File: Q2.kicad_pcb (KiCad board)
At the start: 2 copper layers, 86 x 55 mm, 167 parts, among them U1 LM317, U10 SP-2U1+, U11 SMA, U12 LT1009, U13 TL974, U14 PMA4-33GLN+, U2 Teensy3.2, U3 SMA, U4 ROS-2536C-119+, U5 PMA4-33GLN+, U6 PGA-103+, U7 TCBT-14+, U8 SIM-43LH+, U9 GAT-7+

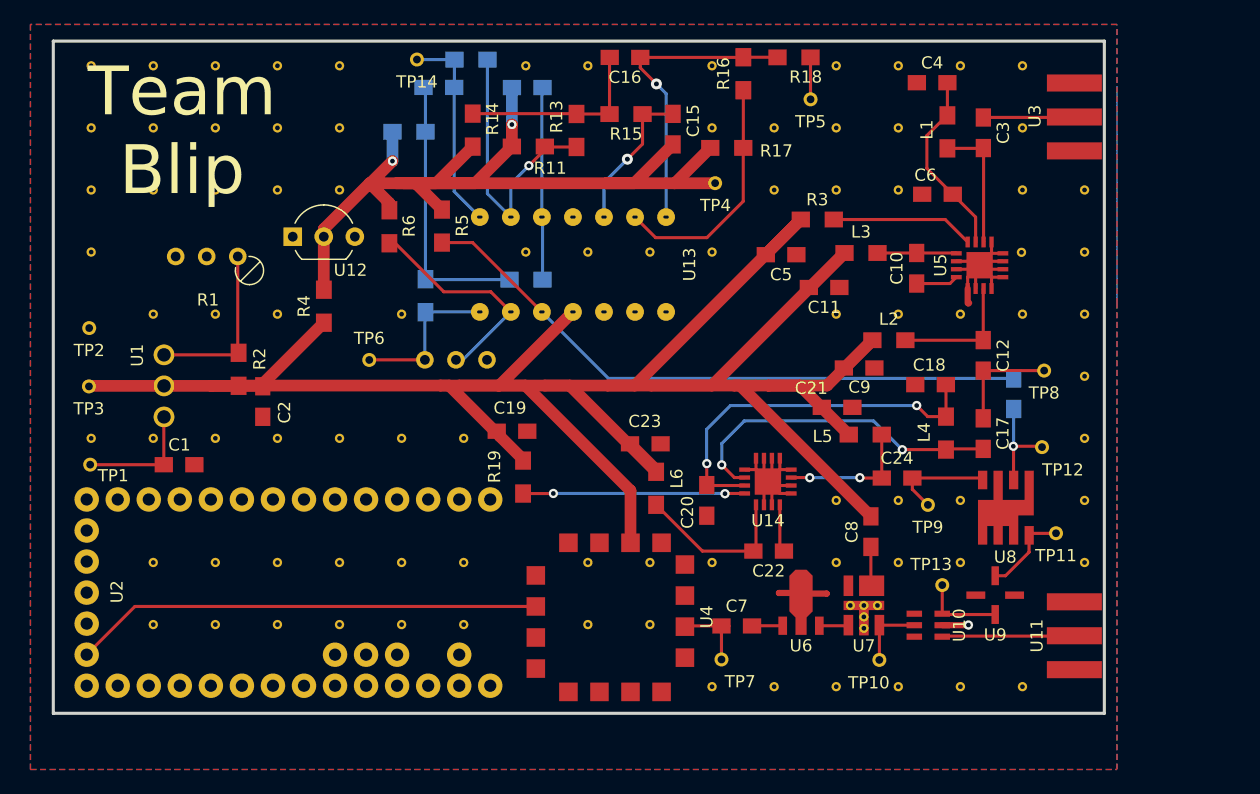
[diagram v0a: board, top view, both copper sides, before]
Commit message: Update
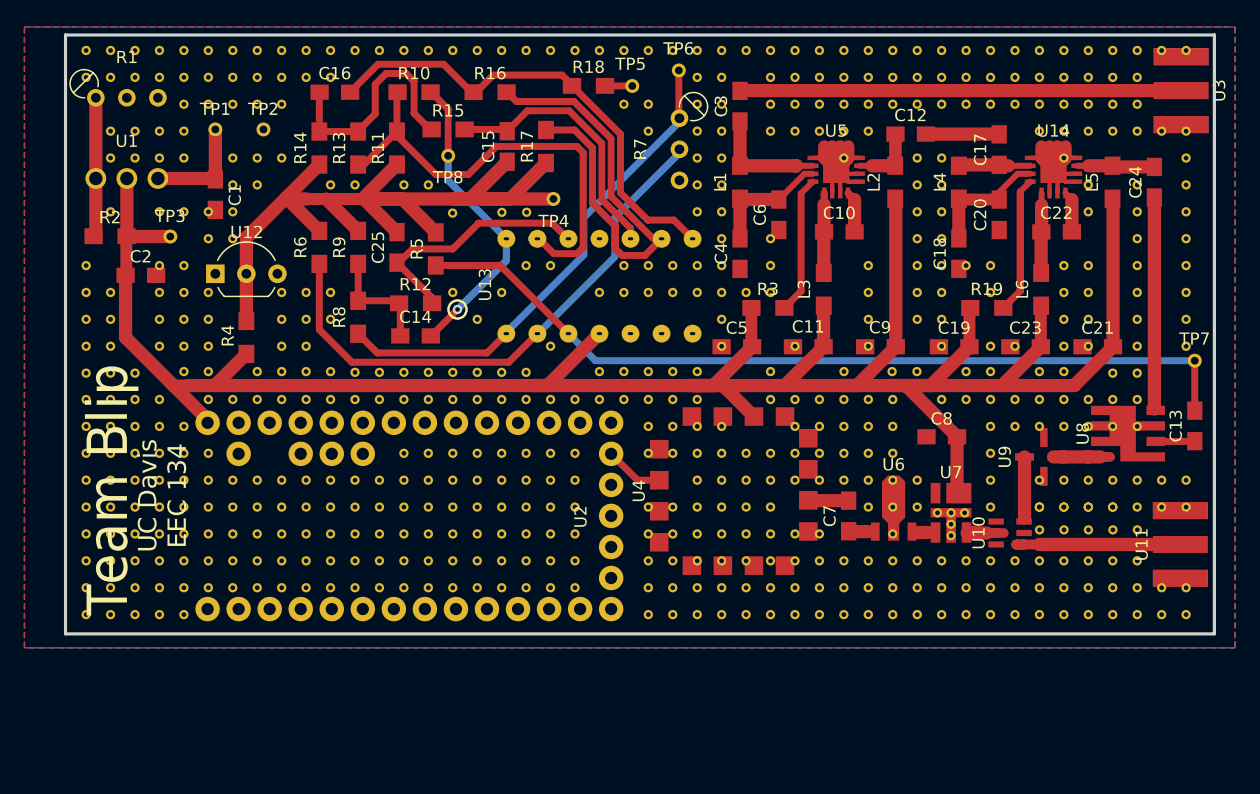
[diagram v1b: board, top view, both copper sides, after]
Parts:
- removed the REF** at (99.1, 53.3)
- removed the REF** at (88.9, 73.7)
- removed the REF** at (88.9, 38.1)
- removed the REF** at (88.9, 33.0)
- removed the REF** at (94.0, 38.1)
- removed the REF** at (104.1, 38.1)
- removed the REF** at (99.1, 38.1)
- removed the REF** at (58.4, 38.1)
- removed the REF** at (99.1, 68.6)
- removed the REF** at (109.2, 68.6)
- removed the REF** at (104.1, 68.6)
- removed the REF** at (104.1, 53.3)
- removed the REF** at (99.1, 73.7)
- removed the REF** at (104.1, 73.7)
- removed the REF** at (109.2, 73.7)
- removed the REF** at (58.4, 78.7)
- removed the REF** at (53.3, 78.7)
- removed the REF** at (48.3, 78.7)
- removed the REF** at (43.2, 78.7)
- removed the REF** at (43.2, 73.7)
- removed the REF** at (48.3, 73.7)
- removed the REF** at (53.3, 73.7)
- removed the REF** at (109.2, 53.3)
- removed the REF** at (58.4, 73.7)
- removed the REF** at (63.5, 73.7)
- removed the REF** at (63.5, 78.7)
- removed the REF** at (68.6, 73.7)
- removed the REF** at (68.6, 78.7)
- removed the REF** at (78.7, 78.7)
- removed the REF** at (78.7, 73.7)
- removed the REF** at (83.8, 73.7)
- removed the REF** at (83.8, 78.7)
- removed the REF** at (88.9, 83.8)
- removed the REF** at (114.3, 53.3)
- removed the REF** at (94.0, 83.8)
- removed the REF** at (99.1, 83.8)
- removed the REF** at (104.1, 83.8)
- removed the REF** at (109.2, 83.8)
- removed the REF** at (114.3, 83.8)
- removed the REF** at (119.4, 73.7)
- removed the REF** at (119.4, 68.6)
- removed the REF** at (119.4, 63.5)
- removed the REF** at (119.4, 58.4)
- removed the REF** at (119.4, 53.3)
- removed the REF** at (104.1, 43.2)
- removed the REF** at (94.0, 43.2)
- removed the REF** at (119.4, 43.2)
- removed the REF** at (119.4, 48.3)
- removed the REF** at (68.6, 63.5)
- removed the REF** at (63.5, 63.5)
- removed the REF** at (58.4, 63.5)
- removed the REF** at (38.1, 63.5)
- removed the REF** at (43.2, 63.5)
- removed the REF** at (53.3, 63.5)
- removed the REF** at (48.3, 63.5)
- removed the REF** at (99.1, 43.2)
- removed the REF** at (38.1, 38.1)
- removed the REF** at (88.9, 48.3)
- removed the REF** at (83.8, 48.3)
- removed the REF** at (78.7, 48.3)
- removed the REF** at (73.7, 48.3)
- removed the REF** at (114.3, 43.2)
- removed the REF** at (114.3, 38.1)
- removed the REF** at (114.3, 33.0)
- removed the REF** at (109.2, 33.0)
- removed the REF** at (104.1, 33.0)
- removed the REF** at (58.4, 43.2)
- removed the REF** at (99.1, 33.0)
- removed the REF** at (94.0, 33.0)
- removed the REF** at (58.4, 33.0)
- removed the REF** at (53.3, 33.0)
- removed the REF** at (48.3, 33.0)
- removed the REF** at (43.2, 33.0)
- removed the REF** at (38.1, 33.0)
- removed the REF** at (38.1, 43.2)
- removed the REF** at (43.2, 38.1)
- removed the REF** at (48.3, 38.1)
- removed the REF** at (43.2, 53.3)
- removed the REF** at (53.3, 38.1)
- removed the REF** at (43.2, 43.2)
- removed the REF** at (48.3, 43.2)
- removed the REF** at (53.3, 43.2)
- removed the REF** at (53.3, 53.3)
- removed the REF** at (48.3, 53.3)
- removed the REF** at (73.7, 33.0)
- removed the REF** at (78.7, 33.0)
- removed the REF** at (114.2, 48.3)
- removed the REF** at (63.5, 53.3)
- removed the REF** at (38.1, 48.3)
- removed TP10, TP11, TP12, TP13, TP14, TP9: TEST, Q2Footprint:PINTST
- added REF**: via-15mil, Q2Footprint:via-15mil, F.Cu at (75.7, 56.0)
- added REF**: via-15mil, Q2Footprint:via-15mil, F.Cu at (87.7, 34.0)
- added REF**: via-15mil, Q2Footprint:via-15mil, F.Cu at (37.7, 34.0)
- added REF**: via-15mil, Q2Footprint:via-15mil, F.Cu at (39.7, 34.0)
- added REF**: via-15mil, Q2Footprint:via-15mil, F.Cu at (41.7, 34.0)
- added REF**: via-15mil, Q2Footprint:via-15mil, F.Cu at (43.7, 34.0)
- added REF**: via-15mil, Q2Footprint:via-15mil, F.Cu at (45.7, 34.0)
- added REF**: via-15mil, Q2Footprint:via-15mil, F.Cu at (47.7, 34.0)
- added REF**: via-15mil, Q2Footprint:via-15mil, F.Cu at (39.7, 40.6)
- added REF**: via-15mil, Q2Footprint:via-15mil, F.Cu at (41.7, 40.6)
- added REF**: via-15mil, Q2Footprint:via-15mil, F.Cu at (43.7, 40.6)
- added REF**: via-15mil, Q2Footprint:via-15mil, F.Cu at (45.7, 40.6)
- added REF**: via-15mil, Q2Footprint:via-15mil, F.Cu at (89.7, 47.2)
- added REF**: via-15mil, Q2Footprint:via-15mil, F.Cu at (39.7, 45.0)
- added REF**: via-15mil, Q2Footprint:via-15mil, F.Cu at (43.7, 45.0)
- added REF**: via-15mil, Q2Footprint:via-15mil, F.Cu at (45.7, 45.0)
- added REF**: via-15mil, Q2Footprint:via-15mil, F.Cu at (47.7, 47.2)
- added REF**: via-15mil, Q2Footprint:via-15mil, F.Cu at (49.7, 47.2)
- added REF**: via-15mil, Q2Footprint:via-15mil, F.Cu at (49.7, 45.0)
- added REF**: via-15mil, Q2Footprint:via-15mil, F.Cu at (49.7, 42.8)
- added REF**: via-15mil, Q2Footprint:via-15mil, F.Cu at (49.7, 40.6)
- added REF**: via-15mil, Q2Footprint:via-15mil, F.Cu at (49.7, 36.2)
- added REF**: via-15mil, Q2Footprint:via-15mil, F.Cu at (49.7, 34.0)
- added REF**: via-15mil, Q2Footprint:via-15mil, F.Cu at (47.7, 45.0)
- added REF**: via-15mil, Q2Footprint:via-15mil, F.Cu at (91.7, 51.6)
- added REF**: via-15mil, Q2Footprint:via-15mil, F.Cu at (89.7, 51.6)
- added REF**: via-15mil, Q2Footprint:via-15mil, F.Cu at (87.7, 51.6)
- added REF**: via-15mil, Q2Footprint:via-15mil, F.Cu at (85.7, 51.6)
- added REF**: via-15mil, Q2Footprint:via-15mil, F.Cu at (83.7, 51.6)
- added REF**: via-15mil, Q2Footprint:via-15mil, F.Cu at (81.7, 51.6)
- added REF**: via-15mil, Q2Footprint:via-15mil, F.Cu at (79.7, 51.6)
- added REF**: via-15mil, Q2Footprint:via-15mil, F.Cu at (57.7, 53.8)
- added REF**: via-15mil, Q2Footprint:via-15mil, F.Cu at (71.7, 51.6)
- added REF**: via-15mil, Q2Footprint:via-15mil, F.Cu at (67.7, 51.6)
- added REF**: via-15mil, Q2Footprint:via-15mil, F.Cu at (69.7, 53.8)
- added REF**: via-15mil, Q2Footprint:via-15mil, F.Cu at (57.7, 51.6)
- added REF**: via-15mil, Q2Footprint:via-15mil, F.Cu at (37.7, 31.8)
- added REF**: via-15mil, Q2Footprint:via-15mil, F.Cu at (39.7, 31.8)
- added REF**: via-15mil, Q2Footprint:via-15mil, F.Cu at (41.7, 31.8)
- added REF**: via-15mil, Q2Footprint:via-15mil, F.Cu at (43.7, 31.8)
- added REF**: via-15mil, Q2Footprint:via-15mil, F.Cu at (45.7, 31.8)
- added REF**: via-15mil, Q2Footprint:via-15mil, F.Cu at (47.7, 31.8)
- added REF**: via-15mil, Q2Footprint:via-15mil, F.Cu at (49.7, 31.8)
- added REF**: via-15mil, Q2Footprint:via-15mil, F.Cu at (51.7, 31.8)
- added REF**: via-15mil, Q2Footprint:via-15mil, F.Cu at (53.7, 31.8)
- added REF**: via-15mil, Q2Footprint:via-15mil, F.Cu at (75.7, 49.4)
- added REF**: via-15mil, Q2Footprint:via-15mil, F.Cu at (55.7, 31.8)
- added REF**: via-15mil, Q2Footprint:via-15mil, F.Cu at (57.7, 31.8)
- added REF**: via-15mil, Q2Footprint:via-15mil, F.Cu at (59.7, 31.8)
- added REF**: via-15mil, Q2Footprint:via-15mil, F.Cu at (61.7, 31.8)
- added REF**: via-15mil, Q2Footprint:via-15mil, F.Cu at (63.7, 31.8)
- added REF**: via-15mil, Q2Footprint:via-15mil, F.Cu at (65.7, 31.8)
- added REF**: via-15mil, Q2Footprint:via-15mil, F.Cu at (67.7, 31.8)
- added REF**: via-15mil, Q2Footprint:via-15mil, F.Cu at (69.7, 31.8)
- added REF**: via-15mil, Q2Footprint:via-15mil, F.Cu at (71.7, 31.8)
- added REF**: via-15mil, Q2Footprint:via-15mil, F.Cu at (73.7, 31.8)
- added REF**: via-15mil, Q2Footprint:via-15mil, F.Cu at (73.7, 49.4)
- added REF**: via-15mil, Q2Footprint:via-15mil, F.Cu at (75.7, 31.8)
- added REF**: via-15mil, Q2Footprint:via-15mil, F.Cu at (77.7, 31.8)
- added REF**: via-15mil, Q2Footprint:via-15mil, F.Cu at (79.7, 31.8)
- added REF**: via-15mil, Q2Footprint:via-15mil, F.Cu at (81.7, 31.8)
- added REF**: via-15mil, Q2Footprint:via-15mil, F.Cu at (83.7, 31.8)
- added REF**: via-15mil, Q2Footprint:via-15mil, F.Cu at (85.7, 31.8)
- added REF**: via-15mil, Q2Footprint:via-15mil, F.Cu at (87.7, 31.8)
- added REF**: via-15mil, Q2Footprint:via-15mil, F.Cu at (71.7, 45.0)
- added REF**: via-15mil, Q2Footprint:via-15mil, F.Cu at (67.7, 45.1)
- added REF**: via-15mil, Q2Footprint:via-15mil, F.Cu at (59.7, 42.8)
- added REF**: via-15mil, Q2Footprint:via-15mil, F.Cu at (73.7, 45.0)
- added REF**: via-15mil, Q2Footprint:via-15mil, F.Cu at (57.7, 42.8)
- added REF**: via-15mil, Q2Footprint:via-15mil, F.Cu at (65.7, 42.8)
- added REF**: via-15mil, Q2Footprint:via-15mil, F.Cu at (63.7, 42.8)
- added REF**: via-15mil, Q2Footprint:via-15mil, F.Cu at (55.7, 51.6)
- added REF**: via-15mil, Q2Footprint:via-15mil, F.Cu at (55.7, 53.8)
- added REF**: via-15mil, Q2Footprint:via-15mil, F.Cu at (55.7, 56.0)
- added REF**: via-15mil, Q2Footprint:via-15mil, F.Cu at (53.7, 51.6)
- added REF**: via-15mil, Q2Footprint:via-15mil, F.Cu at (53.7, 53.8)
- added REF**: via-15mil, Q2Footprint:via-15mil, F.Cu at (53.7, 56.0)
- added REF**: via-15mil, Q2Footprint:via-15mil, F.Cu at (47.7, 51.6)
- added REF**: via-15mil, Q2Footprint:via-15mil, F.Cu at (93.7, 47.2)
- added REF**: via-15mil, Q2Footprint:via-15mil, F.Cu at (47.7, 53.8)
- added REF**: via-15mil, Q2Footprint:via-15mil, F.Cu at (47.7, 56.0)
- added REF**: via-15mil, Q2Footprint:via-15mil, F.Cu at (45.7, 56.0)
- added REF**: via-15mil, Q2Footprint:via-15mil, F.Cu at (45.7, 53.8)
- added REF**: via-15mil, Q2Footprint:via-15mil, F.Cu at (45.7, 51.6)
- added REF**: via-15mil, Q2Footprint:via-15mil, F.Cu at (43.7, 56.0)
- added REF**: via-15mil, Q2Footprint:via-15mil, F.Cu at (43.7, 53.8)
- added REF**: via-15mil, Q2Footprint:via-15mil, F.Cu at (43.7, 51.6)
- added REF**: via-15mil, Q2Footprint:via-15mil, F.Cu at (39.7, 51.6)
- added REF**: via-15mil, Q2Footprint:via-15mil, F.Cu at (39.7, 53.8)
- added REF**: via-15mil, Q2Footprint:via-15mil, F.Cu at (109.7, 49.4)
- added REF**: via-15mil, Q2Footprint:via-15mil, F.Cu at (39.7, 56.0)
- added REF**: via-15mil, Q2Footprint:via-15mil, F.Cu at (45.7, 49.4)
- added REF**: via-15mil, Q2Footprint:via-15mil, F.Cu at (43.7, 49.4)
- added REF**: via-15mil, Q2Footprint:via-15mil, F.Cu at (37.7, 49.4)
- added REF**: via-15mil, Q2Footprint:via-15mil, F.Cu at (37.7, 51.6)
- added REF**: via-15mil, Q2Footprint:via-15mil, F.Cu at (37.7, 53.8)
- added REF**: via-15mil, Q2Footprint:via-15mil, F.Cu at (37.7, 56.0)
- added REF**: via-15mil, Q2Footprint:via-15mil, F.Cu at (107.7, 40.6)
- added REF**: via-15mil, Q2Footprint:via-15mil, F.Cu at (105.7, 40.6)
- added REF**: via-15mil, Q2Footprint:via-15mil, F.Cu at (107.7, 42.8)
- added REF**: via-15mil, Q2Footprint:via-15mil, F.Cu at (113.7, 56.0)
- added REF**: via-15mil, Q2Footprint:via-15mil, F.Cu at (105.7, 42.8)
- added REF**: via-15mil, Q2Footprint:via-15mil, F.Cu at (107.7, 45.0)
- added REF**: via-15mil, Q2Footprint:via-15mil, F.Cu at (105.7, 45.0)
- added REF**: via-15mil, Q2Footprint:via-15mil, F.Cu at (107.7, 47.2)
- added REF**: via-15mil, Q2Footprint:via-15mil, F.Cu at (105.7, 47.2)
- added REF**: via-15mil, Q2Footprint:via-15mil, F.Cu at (105.7, 49.4)
- added REF**: via-15mil, Q2Footprint:via-15mil, F.Cu at (105.7, 51.6)
- added REF**: via-15mil, Q2Footprint:via-15mil, F.Cu at (105.7, 53.8)
- added REF**: via-15mil, Q2Footprint:via-15mil, F.Cu at (107.7, 53.8)
- added REF**: via-15mil, Q2Footprint:via-15mil, F.Cu at (107.7, 51.6)
- added REF**: via-15mil, Q2Footprint:via-15mil, F.Cu at (83.7, 38.4)
- added REF**: via-15mil, Q2Footprint:via-15mil, F.Cu at (119.7, 62.5)
- added REF**: via-15mil, Q2Footprint:via-15mil, F.Cu at (107.7, 49.4)
- added REF**: via-15mil, Q2Footprint:via-15mil, F.Cu at (111.7, 51.6)
- added REF**: via-15mil, Q2Footprint:via-15mil, F.Cu at (111.7, 49.4)
- added REF**: via-15mil, Q2Footprint:via-15mil, F.Cu at (93.7, 36.2)
- added REF**: via-15mil, Q2Footprint:via-15mil, F.Cu at (95.7, 36.2)
- added REF**: via-15mil, Q2Footprint:via-15mil, F.Cu at (97.7, 36.2)
- added REF**: via-15mil, Q2Footprint:via-15mil, F.Cu at (99.7, 36.2)
- added REF**: via-15mil, Q2Footprint:via-15mil, F.Cu at (101.7, 36.2)
- added REF**: via-15mil, Q2Footprint:via-15mil, F.Cu at (103.7, 36.2)
- added REF**: via-15mil, Q2Footprint:via-15mil, F.Cu at (105.7, 36.2)
- added REF**: via-15mil, Q2Footprint:via-15mil, F.Cu at (123.7, 62.5)
- added REF**: via-15mil, Q2Footprint:via-15mil, F.Cu at (107.7, 36.2)
- added REF**: via-15mil, Q2Footprint:via-15mil, F.Cu at (109.7, 36.2)
- added REF**: via-15mil, Q2Footprint:via-15mil, F.Cu at (111.7, 36.2)
- added REF**: via-15mil, Q2Footprint:via-15mil, F.Cu at (113.7, 36.2)
- added REF**: via-15mil, Q2Footprint:via-15mil, F.Cu at (115.7, 36.2)
- added REF**: via-15mil, Q2Footprint:via-15mil, F.Cu at (117.7, 36.2)
- added REF**: via-15mil, Q2Footprint:via-15mil, F.Cu at (119.7, 36.2)
- added REF**: via-15mil, Q2Footprint:via-15mil, F.Cu at (121.7, 36.2)
- added REF**: via-15mil, Q2Footprint:via-15mil, F.Cu at (123.7, 36.2)
- added REF**: via-15mil, Q2Footprint:via-15mil, F.Cu at (119.7, 42.8)
- added REF**: via-15mil, Q2Footprint:via-15mil, F.Cu at (121.7, 62.5)
- added REF**: via-15mil, Q2Footprint:via-15mil, F.Cu at (119.7, 45.0)
- added REF**: via-15mil, Q2Footprint:via-15mil, F.Cu at (111.7, 56.0)
- added REF**: via-15mil, Q2Footprint:via-15mil, F.Cu at (117.7, 49.4)
- added REF**: via-15mil, Q2Footprint:via-15mil, F.Cu at (119.7, 49.4)
- added REF**: via-15mil, Q2Footprint:via-15mil, F.Cu at (117.7, 51.6)
- added REF**: via-15mil, Q2Footprint:via-15mil, F.Cu at (119.7, 51.6)
- added REF**: via-15mil, Q2Footprint:via-15mil, F.Cu at (117.7, 53.8)
- added REF**: via-15mil, Q2Footprint:via-15mil, F.Cu at (119.7, 53.8)
- added REF**: via-15mil, Q2Footprint:via-15mil, F.Cu at (115.7, 38.4)
- added REF**: via-15mil, Q2Footprint:via-15mil, F.Cu at (117.7, 38.4)
- added REF**: via-15mil, Q2Footprint:via-15mil, F.Cu at (103.7, 71.3)
- added REF**: via-15mil, Q2Footprint:via-15mil, F.Cu at (119.7, 38.4)
- added REF**: via-15mil, Q2Footprint:via-15mil, F.Cu at (121.7, 38.4)
- added REF**: via-15mil, Q2Footprint:via-15mil, F.Cu at (89.7, 34.0)
- added REF**: via-15mil, Q2Footprint:via-15mil, F.Cu at (93.7, 34.0)
- added REF**: via-15mil, Q2Footprint:via-15mil, F.Cu at (95.7, 34.0)
- added REF**: via-15mil, Q2Footprint:via-15mil, F.Cu at (97.7, 34.0)
- added REF**: via-15mil, Q2Footprint:via-15mil, F.Cu at (99.7, 34.0)
- added REF**: via-15mil, Q2Footprint:via-15mil, F.Cu at (101.7, 34.0)
- added REF**: via-15mil, Q2Footprint:via-15mil, F.Cu at (103.7, 34.0)
- added REF**: via-15mil, Q2Footprint:via-15mil, F.Cu at (105.7, 34.0)
- added REF**: via-15mil, Q2Footprint:via-15mil, F.Cu at (103.7, 66.9)
- added REF**: via-15mil, Q2Footprint:via-15mil, F.Cu at (107.7, 34.0)
- added REF**: via-15mil, Q2Footprint:via-15mil, F.Cu at (109.7, 34.0)
- added REF**: via-15mil, Q2Footprint:via-15mil, F.Cu at (111.7, 34.0)
- added REF**: via-15mil, Q2Footprint:via-15mil, F.Cu at (113.7, 34.0)
- added REF**: via-15mil, Q2Footprint:via-15mil, F.Cu at (115.7, 34.0)
- added REF**: via-15mil, Q2Footprint:via-15mil, F.Cu at (117.7, 34.0)
- added REF**: via-15mil, Q2Footprint:via-15mil, F.Cu at (119.7, 34.0)
- added REF**: via-15mil, Q2Footprint:via-15mil, F.Cu at (121.7, 34.0)
- added REF**: via-15mil, Q2Footprint:via-15mil, F.Cu at (123.7, 34.0)
- added REF**: via-15mil, Q2Footprint:via-15mil, F.Cu at (89.7, 31.8)
- added REF**: via-15mil, Q2Footprint:via-15mil, F.Cu at (103.7, 69.1)
- added REF**: via-15mil, Q2Footprint:via-15mil, F.Cu at (91.7, 31.8)
- added REF**: via-15mil, Q2Footprint:via-15mil, F.Cu at (93.7, 31.8)
- added REF**: via-15mil, Q2Footprint:via-15mil, F.Cu at (95.7, 31.8)
- added REF**: via-15mil, Q2Footprint:via-15mil, F.Cu at (97.7, 31.8)
- added REF**: via-15mil, Q2Footprint:via-15mil, F.Cu at (99.7, 31.8)
- added REF**: via-15mil, Q2Footprint:via-15mil, F.Cu at (101.7, 31.8)
- added REF**: via-15mil, Q2Footprint:via-15mil, F.Cu at (103.7, 31.8)
- added REF**: via-15mil, Q2Footprint:via-15mil, F.Cu at (105.7, 31.8)
- added REF**: via-15mil, Q2Footprint:via-15mil, F.Cu at (107.7, 31.8)
- added REF**: via-15mil, Q2Footprint:via-15mil, F.Cu at (109.7, 31.8)
- added REF**: via-15mil, Q2Footprint:via-15mil, F.Cu at (115.7, 66.9)
- added REF**: via-15mil, Q2Footprint:via-15mil, F.Cu at (111.7, 31.8)
- added REF**: via-15mil, Q2Footprint:via-15mil, F.Cu at (113.7, 31.8)
- added REF**: via-15mil, Q2Footprint:via-15mil, F.Cu at (115.7, 31.8)
- added REF**: via-15mil, Q2Footprint:via-15mil, F.Cu at (117.7, 31.8)
- added REF**: via-15mil, Q2Footprint:via-15mil, F.Cu at (119.7, 31.8)
- added REF**: via-15mil, Q2Footprint:via-15mil, F.Cu at (121.7, 31.8)
- added REF**: via-15mil, Q2Footprint:via-15mil, F.Cu at (123.7, 31.8)
- added REF**: via-15mil, Q2Footprint:via-15mil, F.Cu at (123.7, 38.4)
- added REF**: via-15mil, Q2Footprint:via-15mil, F.Cu at (123.7, 42.8)
- added REF**: via-15mil, Q2Footprint:via-15mil, F.Cu at (123.7, 45.0)
- added REF**: via-15mil, Q2Footprint:via-15mil, F.Cu at (115.7, 62.5)
- added REF**: via-15mil, Q2Footprint:via-15mil, F.Cu at (123.7, 47.2)
- added REF**: via-15mil, Q2Footprint:via-15mil, F.Cu at (123.7, 49.4)
- added REF**: via-15mil, Q2Footprint:via-15mil, F.Cu at (123.7, 51.6)
- added REF**: via-15mil, Q2Footprint:via-15mil, F.Cu at (123.7, 53.8)
- added REF**: via-15mil, Q2Footprint:via-15mil, F.Cu at (127.7, 40.6)
- added REF**: via-15mil, Q2Footprint:via-15mil, F.Cu at (127.7, 42.8)
- added REF**: via-15mil, Q2Footprint:via-15mil, F.Cu at (127.7, 45.0)
- added REF**: via-15mil, Q2Footprint:via-15mil, F.Cu at (127.7, 47.2)
- added REF**: via-15mil, Q2Footprint:via-15mil, F.Cu at (127.7, 49.4)
- added REF**: via-15mil, Q2Footprint:via-15mil, F.Cu at (127.7, 51.6)
- added REF**: via-15mil, Q2Footprint:via-15mil, F.Cu at (97.7, 71.3)
- added REF**: via-15mil, Q2Footprint:via-15mil, F.Cu at (127.7, 53.8)
- added REF**: via-15mil, Q2Footprint:via-15mil, F.Cu at (127.7, 56.0)
- added REF**: via-15mil, Q2Footprint:via-15mil, F.Cu at (123.7, 56.0)
- added REF**: via-15mil, Q2Footprint:via-15mil, F.Cu at (117.7, 56.0)
- added REF**: via-15mil, Q2Footprint:via-15mil, F.Cu at (127.7, 66.9)
- added REF**: via-15mil, Q2Footprint:via-15mil, F.Cu at (125.7, 66.9)
- added REF**: via-15mil, Q2Footprint:via-15mil, F.Cu at (123.7, 66.9)
- added REF**: via-15mil, Q2Footprint:via-15mil, F.Cu at (121.7, 66.9)
- added REF**: via-15mil, Q2Footprint:via-15mil, F.Cu at (119.7, 66.9)
- added REF**: via-15mil, Q2Footprint:via-15mil, F.Cu at (117.7, 66.9)
- added REF**: via-15mil, Q2Footprint:via-15mil, F.Cu at (95.7, 71.3)
- added REF**: via-15mil, Q2Footprint:via-15mil, F.Cu at (117.7, 62.5)
- added REF**: via-15mil, Q2Footprint:via-15mil, F.Cu at (113.7, 62.5)
- added REF**: via-15mil, Q2Footprint:via-15mil, F.Cu at (111.7, 66.9)
- added REF**: via-15mil, Q2Footprint:via-15mil, F.Cu at (111.7, 64.7)
- added REF**: via-15mil, Q2Footprint:via-15mil, F.Cu at (111.7, 62.5)
- added REF**: via-15mil, Q2Footprint:via-15mil, F.Cu at (103.7, 64.7)
- added REF**: via-15mil, Q2Footprint:via-15mil, F.Cu at (103.7, 62.5)
- added REF**: via-15mil, Q2Footprint:via-15mil, F.Cu at (99.7, 66.9)
- added REF**: via-15mil, Q2Footprint:via-15mil, F.Cu at (99.7, 64.7)
- added REF**: via-15mil, Q2Footprint:via-15mil, F.Cu at (99.7, 62.5)
- added REF**: via-15mil, Q2Footprint:via-15mil, F.Cu at (83.7, 36.2)
- added REF**: via-15mil, Q2Footprint:via-15mil, F.Cu at (87.7, 73.5)
- added REF**: via-15mil, Q2Footprint:via-15mil, F.Cu at (101.7, 62.5)
- added REF**: via-15mil, Q2Footprint:via-15mil, F.Cu at (101.7, 64.7)
- added REF** (x2): via-15mil, Q2Footprint:via-15mil, F.Cu at (121.7, 69.1)
- added REF** (x2): via-15mil, Q2Footprint:via-15mil, F.Cu at (119.7, 69.1)
- added REF** (x2): via-15mil, Q2Footprint:via-15mil, F.Cu at (117.7, 69.1)
- added REF** (x2): via-15mil, Q2Footprint:via-15mil, F.Cu at (115.7, 69.1)
- added REF**: via-15mil, Q2Footprint:via-15mil, F.Cu at (123.7, 71.0)
- added REF**: via-15mil, Q2Footprint:via-15mil, F.Cu at (121.7, 71.0)
- added REF**: via-15mil, Q2Footprint:via-15mil, F.Cu at (119.7, 71.0)
- added REF**: via-15mil, Q2Footprint:via-15mil, F.Cu at (117.7, 71.0)
- added REF**: via-15mil, Q2Footprint:via-15mil, F.Cu at (89.7, 73.5)
- added REF**: via-15mil, Q2Footprint:via-15mil, F.Cu at (115.7, 71.0)
- added REF**: via-15mil, Q2Footprint:via-15mil, F.Cu at (101.7, 66.9)
- added REF**: via-15mil, Q2Footprint:via-15mil, F.Cu at (101.7, 69.1)
- added REF**: via-15mil, Q2Footprint:via-15mil, F.Cu at (105.7, 66.9)
- added REF**: via-15mil, Q2Footprint:via-15mil, F.Cu at (105.7, 69.1)
- added REF**: via-15mil, Q2Footprint:via-15mil, F.Cu at (111.7, 69.1)
- added REF**: via-15mil, Q2Footprint:via-15mil, F.Cu at (123.7, 69.1)
- added REF**: via-15mil, Q2Footprint:via-15mil, F.Cu at (91.7, 73.5)
- added REF**: via-15mil, Q2Footprint:via-15mil, F.Cu at (123.7, 73.5)
- added REF**: via-15mil, Q2Footprint:via-15mil, F.Cu at (121.7, 73.5)
- added REF**: via-15mil, Q2Footprint:via-15mil, F.Cu at (119.7, 73.5)
- added REF**: via-15mil, Q2Footprint:via-15mil, F.Cu at (117.7, 73.5)
- added REF**: via-15mil, Q2Footprint:via-15mil, F.Cu at (115.7, 73.5)
- added REF**: via-15mil, Q2Footprint:via-15mil, F.Cu at (113.7, 73.5)
- added REF**: via-15mil, Q2Footprint:via-15mil, F.Cu at (111.7, 73.5)
- added REF**: via-15mil, Q2Footprint:via-15mil, F.Cu at (109.7, 73.5)
- added REF**: via-15mil, Q2Footprint:via-15mil, F.Cu at (107.7, 73.5)
- added REF**: via-15mil, Q2Footprint:via-15mil, F.Cu at (93.7, 73.5)
- added REF**: via-15mil, Q2Footprint:via-15mil, F.Cu at (105.7, 73.5)
- added REF**: via-15mil, Q2Footprint:via-15mil, F.Cu at (103.7, 73.5)
- added REF**: via-15mil, Q2Footprint:via-15mil, F.Cu at (101.7, 73.5)
- added REF**: via-15mil, Q2Footprint:via-15mil, F.Cu at (99.7, 73.5)
- added REF**: via-15mil, Q2Footprint:via-15mil, F.Cu at (97.7, 73.5)
- added REF**: via-15mil, Q2Footprint:via-15mil, F.Cu at (127.7, 77.9)
- added REF**: via-15mil, Q2Footprint:via-15mil, F.Cu at (125.7, 77.9)
- added REF**: via-15mil, Q2Footprint:via-15mil, F.Cu at (123.7, 77.9)
- added REF**: via-15mil, Q2Footprint:via-15mil, F.Cu at (121.7, 77.9)
- added REF**: via-15mil, Q2Footprint:via-15mil, F.Cu at (119.7, 77.9)
- added REF**: via-15mil, Q2Footprint:via-15mil, F.Cu at (95.7, 73.5)
- added REF**: via-15mil, Q2Footprint:via-15mil, F.Cu at (117.7, 77.9)
- added REF**: via-15mil, Q2Footprint:via-15mil, F.Cu at (115.7, 77.9)
- added REF**: via-15mil, Q2Footprint:via-15mil, F.Cu at (113.7, 77.9)
- added REF**: via-15mil, Q2Footprint:via-15mil, F.Cu at (111.7, 77.9)
- added REF**: via-15mil, Q2Footprint:via-15mil, F.Cu at (109.7, 77.9)
- added REF**: via-15mil, Q2Footprint:via-15mil, F.Cu at (107.7, 77.9)
- added REF**: via-15mil, Q2Footprint:via-15mil, F.Cu at (105.7, 77.9)
- added REF**: via-15mil, Q2Footprint:via-15mil, F.Cu at (103.7, 77.9)
- added REF**: via-15mil, Q2Footprint:via-15mil, F.Cu at (101.7, 77.9)
- added REF**: via-15mil, Q2Footprint:via-15mil, F.Cu at (99.7, 77.9)
- added REF**: via-15mil, Q2Footprint:via-15mil, F.Cu at (95.7, 66.9)
- added REF**: via-15mil, Q2Footprint:via-15mil, F.Cu at (97.7, 77.9)
- added REF**: via-15mil, Q2Footprint:via-15mil, F.Cu at (95.7, 77.9)
- added REF**: via-15mil, Q2Footprint:via-15mil, F.Cu at (93.7, 77.9)
- added REF**: via-15mil, Q2Footprint:via-15mil, F.Cu at (91.7, 77.9)
- added REF**: via-15mil, Q2Footprint:via-15mil, F.Cu at (89.7, 77.9)
- added REF**: via-15mil, Q2Footprint:via-15mil, F.Cu at (123.7, 75.7)
- added REF**: via-15mil, Q2Footprint:via-15mil, F.Cu at (121.7, 75.7)
- added REF**: via-15mil, Q2Footprint:via-15mil, F.Cu at (119.7, 75.7)
- added REF**: via-15mil, Q2Footprint:via-15mil, F.Cu at (117.7, 75.7)
- added REF**: via-15mil, Q2Footprint:via-15mil, F.Cu at (115.7, 75.7)
- added REF**: via-15mil, Q2Footprint:via-15mil, F.Cu at (97.7, 66.9)
- added REF**: via-15mil, Q2Footprint:via-15mil, F.Cu at (113.7, 75.7)
- added REF**: via-15mil, Q2Footprint:via-15mil, F.Cu at (111.7, 75.7)
- added REF**: via-15mil, Q2Footprint:via-15mil, F.Cu at (109.7, 75.7)
- added REF**: via-15mil, Q2Footprint:via-15mil, F.Cu at (107.7, 75.7)
- added REF**: via-15mil, Q2Footprint:via-15mil, F.Cu at (105.7, 75.7)
- added REF**: via-15mil, Q2Footprint:via-15mil, F.Cu at (103.7, 75.7)
- added REF**: via-15mil, Q2Footprint:via-15mil, F.Cu at (101.7, 75.7)
- added REF**: via-15mil, Q2Footprint:via-15mil, F.Cu at (99.7, 75.7)
- added REF**: via-15mil, Q2Footprint:via-15mil, F.Cu at (97.7, 75.7)
- added REF**: via-15mil, Q2Footprint:via-15mil, F.Cu at (95.7, 75.7)
- added REF**: via-15mil, Q2Footprint:via-15mil, F.Cu at (95.7, 64.7)
- added REF**: via-15mil, Q2Footprint:via-15mil, F.Cu at (93.7, 75.7)
- added REF**: via-15mil, Q2Footprint:via-15mil, F.Cu at (91.7, 75.7)
- added REF**: via-15mil, Q2Footprint:via-15mil, F.Cu at (89.7, 75.7)
- added REF**: via-15mil, Q2Footprint:via-15mil, F.Cu at (85.7, 73.5)
- added REF**: via-15mil, Q2Footprint:via-15mil, F.Cu at (83.7, 73.5)
- added REF**: via-15mil, Q2Footprint:via-15mil, F.Cu at (85.7, 62.5)
- added REF**: via-15mil, Q2Footprint:via-15mil, F.Cu at (83.7, 62.5)
- added REF**: via-15mil, Q2Footprint:via-15mil, F.Cu at (93.7, 71.3)
- added REF**: via-15mil, Q2Footprint:via-15mil, F.Cu at (91.7, 71.3)
- added REF**: via-15mil, Q2Footprint:via-15mil, F.Cu at (89.7, 71.3)
- added REF**: via-15mil, Q2Footprint:via-15mil, F.Cu at (97.7, 64.7)
- added REF**: via-15mil, Q2Footprint:via-15mil, F.Cu at (93.7, 69.1)
- added REF**: via-15mil, Q2Footprint:via-15mil, F.Cu at (91.7, 69.1)
- added REF**: via-15mil, Q2Footprint:via-15mil, F.Cu at (89.7, 69.1)
- added REF**: via-15mil, Q2Footprint:via-15mil, F.Cu at (93.7, 66.9)
- added REF**: via-15mil, Q2Footprint:via-15mil, F.Cu at (91.7, 66.9)
- added REF**: via-15mil, Q2Footprint:via-15mil, F.Cu at (89.7, 66.9)
- added REF**: via-15mil, Q2Footprint:via-15mil, F.Cu at (93.7, 64.7)
- added REF**: via-15mil, Q2Footprint:via-15mil, F.Cu at (91.7, 64.7)
- added REF**: via-15mil, Q2Footprint:via-15mil, F.Cu at (89.7, 64.7)
- added REF**: via-15mil, Q2Footprint:via-15mil, F.Cu at (83.7, 77.9)
- added REF**: via-15mil, Q2Footprint:via-15mil, F.Cu at (95.7, 62.5)
- added REF**: via-15mil, Q2Footprint:via-15mil, F.Cu at (85.7, 77.9)
- added REF**: via-15mil, Q2Footprint:via-15mil, F.Cu at (83.7, 75.7)
- added REF**: via-15mil, Q2Footprint:via-15mil, F.Cu at (85.7, 75.7)
- added REF**: via-15mil, Q2Footprint:via-15mil, F.Cu at (87.7, 77.9)
- added REF**: via-15mil, Q2Footprint:via-15mil, F.Cu at (87.7, 75.7)
- added REF**: via-15mil, Q2Footprint:via-15mil, F.Cu at (87.7, 71.3)
- added REF**: via-15mil, Q2Footprint:via-15mil, F.Cu at (87.7, 69.1)
- added REF**: via-15mil, Q2Footprint:via-15mil, F.Cu at (87.7, 66.9)
- added REF**: via-15mil, Q2Footprint:via-15mil, F.Cu at (87.7, 64.7)
- added REF**: via-15mil, Q2Footprint:via-15mil, F.Cu at (77.7, 64.7)
- added REF**: via-15mil, Q2Footprint:via-15mil, F.Cu at (81.7, 36.2)
- added REF**: via-15mil, Q2Footprint:via-15mil, F.Cu at (97.7, 62.5)
- added REF**: via-15mil, Q2Footprint:via-15mil, F.Cu at (75.7, 64.7)
- added REF**: via-15mil, Q2Footprint:via-15mil, F.Cu at (73.7, 64.7)
- added REF**: via-15mil, Q2Footprint:via-15mil, F.Cu at (71.7, 64.7)
- added REF**: via-15mil, Q2Footprint:via-15mil, F.Cu at (69.7, 64.7)
- added REF**: via-15mil, Q2Footprint:via-15mil, F.Cu at (67.7, 64.7)
- added REF**: via-15mil, Q2Footprint:via-15mil, F.Cu at (65.7, 64.7)
- added REF**: via-15mil, Q2Footprint:via-15mil, F.Cu at (63.7, 64.7)
- added REF**: via-15mil, Q2Footprint:via-15mil, F.Cu at (45.7, 77.9)
- added REF**: via-15mil, Q2Footprint:via-15mil, F.Cu at (43.7, 77.9)
- added REF**: via-15mil, Q2Footprint:via-15mil, F.Cu at (41.7, 77.9)
- added REF**: via-15mil, Q2Footprint:via-15mil, F.Cu at (89.7, 62.5)
- added REF**: via-15mil, Q2Footprint:via-15mil, F.Cu at (39.7, 77.9)
- added REF**: via-15mil, Q2Footprint:via-15mil, F.Cu at (77.7, 75.7)
- added REF**: via-15mil, Q2Footprint:via-15mil, F.Cu at (75.7, 75.7)
- added REF**: via-15mil, Q2Footprint:via-15mil, F.Cu at (73.7, 75.7)
- added REF**: via-15mil, Q2Footprint:via-15mil, F.Cu at (71.7, 75.7)
- added REF**: via-15mil, Q2Footprint:via-15mil, F.Cu at (69.7, 75.7)
- added REF**: via-15mil, Q2Footprint:via-15mil, F.Cu at (67.7, 75.7)
- added REF**: via-15mil, Q2Footprint:via-15mil, F.Cu at (65.7, 75.7)
- added REF**: via-15mil, Q2Footprint:via-15mil, F.Cu at (63.7, 75.7)
- added REF**: via-15mil, Q2Footprint:via-15mil, F.Cu at (61.7, 75.7)
- added REF**: via-15mil, Q2Footprint:via-15mil, F.Cu at (87.7, 62.5)
- added REF**: via-15mil, Q2Footprint:via-15mil, F.Cu at (59.7, 75.7)
- added REF**: via-15mil, Q2Footprint:via-15mil, F.Cu at (57.7, 75.7)
- added REF**: via-15mil, Q2Footprint:via-15mil, F.Cu at (55.7, 75.7)
- added REF**: via-15mil, Q2Footprint:via-15mil, F.Cu at (53.7, 75.7)
- added REF**: via-15mil, Q2Footprint:via-15mil, F.Cu at (51.7, 75.7)
- added REF**: via-15mil, Q2Footprint:via-15mil, F.Cu at (49.7, 75.7)
- added REF**: via-15mil, Q2Footprint:via-15mil, F.Cu at (47.7, 75.7)
- added REF**: via-15mil, Q2Footprint:via-15mil, F.Cu at (45.7, 75.7)
- added REF**: via-15mil, Q2Footprint:via-15mil, F.Cu at (43.7, 75.7)
- added REF**: via-15mil, Q2Footprint:via-15mil, F.Cu at (41.7, 75.7)
- added REF**: via-15mil, Q2Footprint:via-15mil, F.Cu at (83.7, 71.3)
- added REF**: via-15mil, Q2Footprint:via-15mil, F.Cu at (39.7, 75.7)
- added REF**: via-15mil, Q2Footprint:via-15mil, F.Cu at (77.7, 73.5)
- added REF**: via-15mil, Q2Footprint:via-15mil, F.Cu at (75.7, 73.5)
- added REF**: via-15mil, Q2Footprint:via-15mil, F.Cu at (73.7, 73.5)
- added REF**: via-15mil, Q2Footprint:via-15mil, F.Cu at (71.7, 73.5)
- added REF**: via-15mil, Q2Footprint:via-15mil, F.Cu at (69.7, 73.5)
- added REF**: via-15mil, Q2Footprint:via-15mil, F.Cu at (67.7, 73.5)
- added REF**: via-15mil, Q2Footprint:via-15mil, F.Cu at (65.7, 73.5)
- added REF**: via-15mil, Q2Footprint:via-15mil, F.Cu at (63.7, 73.5)
- added REF**: via-15mil, Q2Footprint:via-15mil, F.Cu at (61.7, 73.5)
- added REF**: via-15mil, Q2Footprint:via-15mil, F.Cu at (85.7, 71.3)
- added REF**: via-15mil, Q2Footprint:via-15mil, F.Cu at (59.7, 73.5)
- added REF**: via-15mil, Q2Footprint:via-15mil, F.Cu at (57.7, 73.5)
- added REF**: via-15mil, Q2Footprint:via-15mil, F.Cu at (55.7, 73.5)
- added REF**: via-15mil, Q2Footprint:via-15mil, F.Cu at (53.7, 73.5)
- added REF**: via-15mil, Q2Footprint:via-15mil, F.Cu at (51.7, 73.5)
- added REF**: via-15mil, Q2Footprint:via-15mil, F.Cu at (49.7, 73.5)
- added REF**: via-15mil, Q2Footprint:via-15mil, F.Cu at (47.7, 73.5)
- added REF**: via-15mil, Q2Footprint:via-15mil, F.Cu at (45.7, 73.5)
- added REF**: via-15mil, Q2Footprint:via-15mil, F.Cu at (43.7, 73.5)
- added REF**: via-15mil, Q2Footprint:via-15mil, F.Cu at (41.7, 73.5)
- added REF**: via-15mil, Q2Footprint:via-15mil, F.Cu at (83.7, 69.1)
- added REF**: via-15mil, Q2Footprint:via-15mil, F.Cu at (39.7, 73.5)
- added REF**: via-15mil, Q2Footprint:via-15mil, F.Cu at (77.7, 71.3)
- added REF**: via-15mil, Q2Footprint:via-15mil, F.Cu at (75.7, 71.3)
- added REF**: via-15mil, Q2Footprint:via-15mil, F.Cu at (73.7, 71.3)
- added REF**: via-15mil, Q2Footprint:via-15mil, F.Cu at (71.7, 71.3)
- added REF**: via-15mil, Q2Footprint:via-15mil, F.Cu at (69.7, 71.3)
- added REF**: via-15mil, Q2Footprint:via-15mil, F.Cu at (67.7, 71.3)
- added REF**: via-15mil, Q2Footprint:via-15mil, F.Cu at (65.7, 71.3)
- added REF**: via-15mil, Q2Footprint:via-15mil, F.Cu at (63.7, 71.3)
- added REF**: via-15mil, Q2Footprint:via-15mil, F.Cu at (61.7, 71.3)
- added REF**: via-15mil, Q2Footprint:via-15mil, F.Cu at (85.7, 69.1)
- added REF**: via-15mil, Q2Footprint:via-15mil, F.Cu at (59.7, 71.3)
- added REF**: via-15mil, Q2Footprint:via-15mil, F.Cu at (57.7, 71.3)
- added REF**: via-15mil, Q2Footprint:via-15mil, F.Cu at (55.7, 71.3)
- added REF**: via-15mil, Q2Footprint:via-15mil, F.Cu at (53.7, 71.3)
- added REF**: via-15mil, Q2Footprint:via-15mil, F.Cu at (51.7, 71.3)
- added REF**: via-15mil, Q2Footprint:via-15mil, F.Cu at (49.7, 71.3)
- added REF**: via-15mil, Q2Footprint:via-15mil, F.Cu at (47.7, 71.3)
- added REF**: via-15mil, Q2Footprint:via-15mil, F.Cu at (45.7, 71.3)
- added REF**: via-15mil, Q2Footprint:via-15mil, F.Cu at (43.7, 71.3)
- added REF**: via-15mil, Q2Footprint:via-15mil, F.Cu at (41.7, 71.3)
- added REF**: via-15mil, Q2Footprint:via-15mil, F.Cu at (83.7, 64.7)
- added REF**: via-15mil, Q2Footprint:via-15mil, F.Cu at (39.7, 71.3)
- added REF**: via-15mil, Q2Footprint:via-15mil, F.Cu at (77.7, 69.1)
- added REF**: via-15mil, Q2Footprint:via-15mil, F.Cu at (75.7, 69.1)
- added REF**: via-15mil, Q2Footprint:via-15mil, F.Cu at (73.7, 69.1)
- added REF**: via-15mil, Q2Footprint:via-15mil, F.Cu at (71.7, 69.1)
- added REF**: via-15mil, Q2Footprint:via-15mil, F.Cu at (69.7, 69.1)
- added REF**: via-15mil, Q2Footprint:via-15mil, F.Cu at (67.7, 69.1)
- added REF**: via-15mil, Q2Footprint:via-15mil, F.Cu at (65.7, 69.1)
- added REF**: via-15mil, Q2Footprint:via-15mil, F.Cu at (63.7, 69.1)
- added REF**: via-15mil, Q2Footprint:via-15mil, F.Cu at (61.7, 69.1)
- added REF**: via-15mil, Q2Footprint:via-15mil, F.Cu at (85.7, 64.7)
- added REF**: via-15mil, Q2Footprint:via-15mil, F.Cu at (59.7, 69.1)
- added REF**: via-15mil, Q2Footprint:via-15mil, F.Cu at (57.7, 69.1)
- added REF**: via-15mil, Q2Footprint:via-15mil, F.Cu at (55.7, 69.1)
- added REF**: via-15mil, Q2Footprint:via-15mil, F.Cu at (53.7, 69.1)
- added REF**: via-15mil, Q2Footprint:via-15mil, F.Cu at (51.7, 69.1)
- added REF**: via-15mil, Q2Footprint:via-15mil, F.Cu at (49.7, 69.1)
- added REF**: via-15mil, Q2Footprint:via-15mil, F.Cu at (47.7, 69.1)
- added REF**: via-15mil, Q2Footprint:via-15mil, F.Cu at (45.7, 69.1)
- added REF**: via-15mil, Q2Footprint:via-15mil, F.Cu at (43.7, 69.1)
- added REF**: via-15mil, Q2Footprint:via-15mil, F.Cu at (41.7, 69.1)
- added REF**: via-15mil, Q2Footprint:via-15mil, F.Cu at (95.7, 56.0)
- added REF**: via-15mil, Q2Footprint:via-15mil, F.Cu at (39.7, 69.1)
- added REF**: via-15mil, Q2Footprint:via-15mil, F.Cu at (77.7, 66.9)
- added REF**: via-15mil, Q2Footprint:via-15mil, F.Cu at (75.7, 66.9)
- added REF**: via-15mil, Q2Footprint:via-15mil, F.Cu at (73.7, 66.9)
- added REF**: via-15mil, Q2Footprint:via-15mil, F.Cu at (71.7, 66.9)
- added REF**: via-15mil, Q2Footprint:via-15mil, F.Cu at (69.7, 66.9)
- added REF**: via-15mil, Q2Footprint:via-15mil, F.Cu at (67.7, 66.9)
- added REF**: via-15mil, Q2Footprint:via-15mil, F.Cu at (65.7, 66.9)
- added REF**: via-15mil, Q2Footprint:via-15mil, F.Cu at (63.7, 66.9)
- added REF**: via-15mil, Q2Footprint:via-15mil, F.Cu at (61.7, 66.9)
- added REF**: via-15mil, Q2Footprint:via-15mil, F.Cu at (87.7, 45.0)
- added REF**: via-15mil, Q2Footprint:via-15mil, F.Cu at (89.7, 56.0)
- added REF**: via-15mil, Q2Footprint:via-15mil, F.Cu at (59.7, 66.9)
- added REF**: via-15mil, Q2Footprint:via-15mil, F.Cu at (57.7, 66.9)
- added REF**: via-15mil, Q2Footprint:via-15mil, F.Cu at (55.7, 66.9)
- added REF**: via-15mil, Q2Footprint:via-15mil, F.Cu at (53.7, 66.9)
- added REF**: via-15mil, Q2Footprint:via-15mil, F.Cu at (51.7, 66.9)
- added REF**: via-15mil, Q2Footprint:via-15mil, F.Cu at (49.7, 66.9)
- added REF**: via-15mil, Q2Footprint:via-15mil, F.Cu at (47.7, 66.9)
- added REF**: via-15mil, Q2Footprint:via-15mil, F.Cu at (45.7, 66.9)
- added REF**: via-15mil, Q2Footprint:via-15mil, F.Cu at (43.7, 66.9)
- added REF**: via-15mil, Q2Footprint:via-15mil, F.Cu at (41.7, 66.9)
- added REF**: via-15mil, Q2Footprint:via-15mil, F.Cu at (101.7, 56.0)
- added REF**: via-15mil, Q2Footprint:via-15mil, F.Cu at (39.7, 66.9)
- added REF**: via-15mil, Q2Footprint:via-15mil, F.Cu at (37.7, 77.9)
- added REF**: via-15mil, Q2Footprint:via-15mil, F.Cu at (37.7, 75.7)
- added REF**: via-15mil, Q2Footprint:via-15mil, F.Cu at (37.7, 73.5)
- added REF**: via-15mil, Q2Footprint:via-15mil, F.Cu at (37.7, 71.3)
- added REF**: via-15mil, Q2Footprint:via-15mil, F.Cu at (37.7, 69.1)
- added REF**: via-15mil, Q2Footprint:via-15mil, F.Cu at (37.7, 66.9)
- added REF**: via-15mil, Q2Footprint:via-15mil, F.Cu at (47.7, 64.7)
- added REF**: via-15mil, Q2Footprint:via-15mil, F.Cu at (45.7, 64.7)
- added REF**: via-15mil, Q2Footprint:via-15mil, F.Cu at (43.7, 64.7)
- added REF**: via-15mil, Q2Footprint:via-15mil, F.Cu at (107.7, 56.0)
- added REF**: via-15mil, Q2Footprint:via-15mil, F.Cu at (41.7, 64.7)
- added REF**: via-15mil, Q2Footprint:via-15mil, F.Cu at (39.7, 64.7)
- added REF**: via-15mil, Q2Footprint:via-15mil, F.Cu at (37.7, 64.7)
- added REF**: via-15mil, Q2Footprint:via-15mil, F.Cu at (45.7, 62.5)
- added REF**: via-15mil, Q2Footprint:via-15mil, F.Cu at (43.7, 62.5)
- added REF**: via-15mil, Q2Footprint:via-15mil, F.Cu at (41.7, 62.5)
- added REF**: via-15mil, Q2Footprint:via-15mil, F.Cu at (39.7, 62.5)
- added REF**: via-15mil, Q2Footprint:via-15mil, F.Cu at (37.7, 62.5)
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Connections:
- C8 pad 1: Net-(C8-Pad1) -> /+5V
- C8 pad 2: /+5V -> GND
- TP7 pad 1: Net-(C7-Pad2) -> Net-(C13-Pad1)
- TP8 pad 1: Net-(C12-Pad1) -> Net-(C14-Pad2)
- U2 pad 32: Net-(U2-Pad32) -> /+5V
- U7 pad : (no net) -> GND
- U7 pad 3: Net-(C8-Pad1) -> /+5V
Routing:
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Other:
- board size 86 x 55 mm -> 94 x 49 mm
- net class Default: trace_width 0.508 -> 0.572
- net class Fat added: clearance 0.1524, trace_width 1.08408, via_dia 0.762, via_drill 0.381
- net class LNA added: clearance 0.1524, trace_width 1.08408, via_dia 0.762, via_drill 0.381
- rule trace_min: 0.1524 -> 0.1778
- board text added: "UC Davis EEC 134"
